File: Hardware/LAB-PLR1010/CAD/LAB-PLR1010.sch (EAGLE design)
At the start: 7 parts, among them U1 AD5270BRMZ-50, U2 LT3080EMS8EPBF

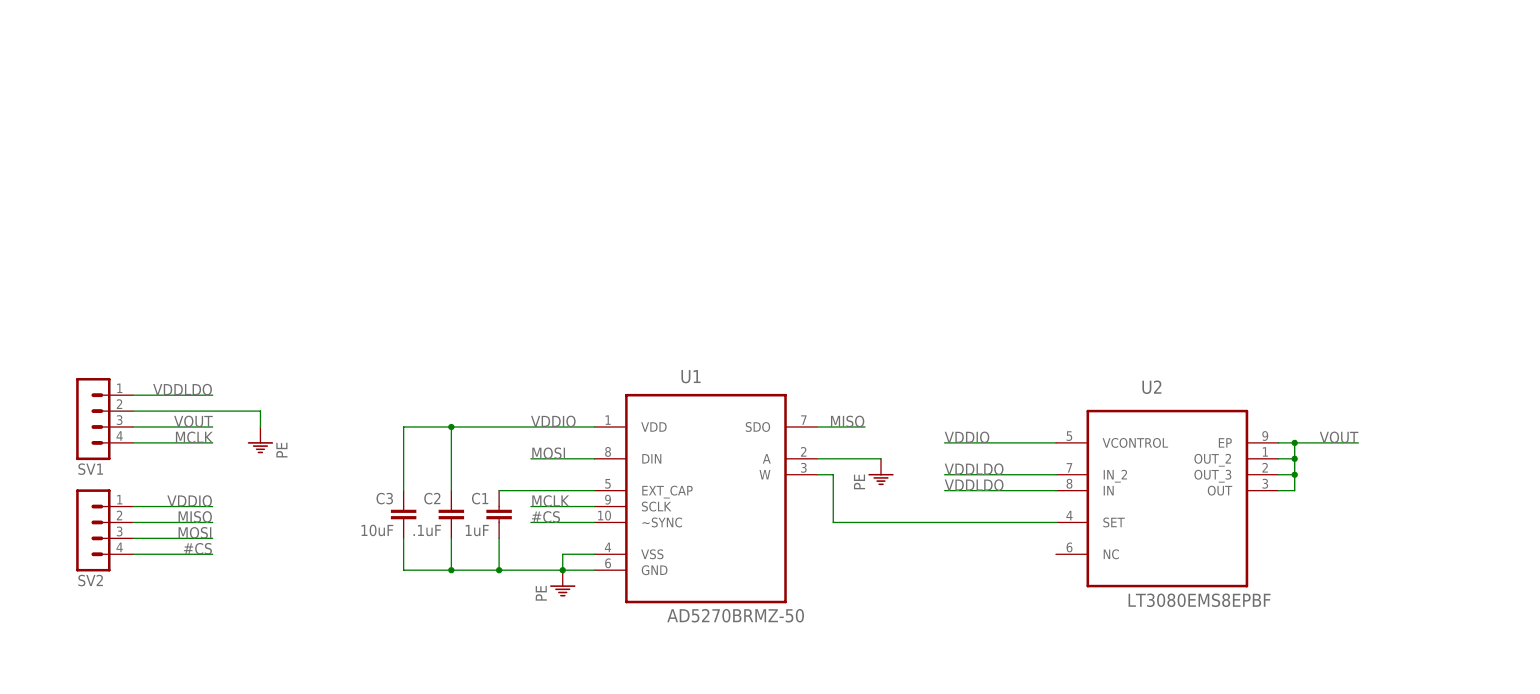
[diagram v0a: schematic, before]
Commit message: 1) Updates to the PLR1010 + datasheet and bills of materials
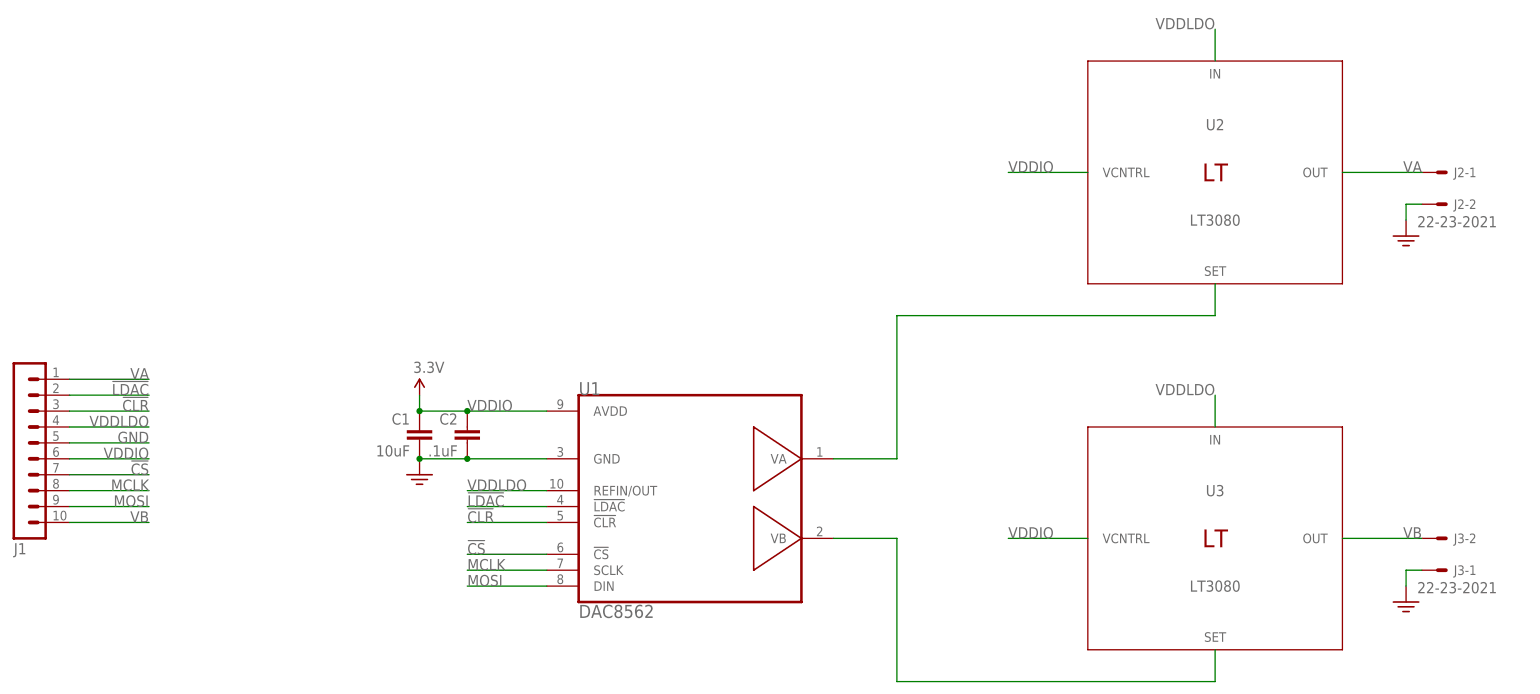
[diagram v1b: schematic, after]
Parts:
- removed C3: 10uF, SparkFun-Capacitors:1NF/1000PF-50V-10%(0603)
- removed SV1, SV2: (no value), LAB304:MA04-1
- added J1: (no value), con-lstb:MA10-1W
- added J2, J3: 22-23-2021, My Library-adm:22-23-2021
- added U3: LT3080, LAB-PLR1010:LT3080
- C1: value 1uF -> 10uF
- U1: value AD5270BRMZ-50 -> DAC8562; device Analog Devices_By_element14_Batch_1:AD5270BRMZ-50 -> LAB-PLR1010:DAC8562
- U2: value LT3080EMS8EPBF -> LT3080; device LAB-PLR1010:LT3080EMS8EPBF -> LAB-PLR1010:LT3080
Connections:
- removed net #CS: SV2.4, U1.~SYNC
- removed net MISO: SV2.2, U1.SDO
- removed net N$1: C1.1, U1.EXT_CAP
- removed net N$8: U1.W, U2.SET
- removed net PE: C1.2, C2.2, C3.2, SV1.2, U1.A, U1.GND, U1.VSS
- removed net VOUT: SV1.3, U2.EP, U2.OUT, U2.OUT_2, U2.OUT_3
- new net !CLR: J1.3, U1.!CLR
- new net !CS: J1.7, U1.!CS
- new net !LDAC: J1.2, U1.!LDAC
- new net GND: C1.2, C2.2, J1.5, J2-2.S, J3-1.S, U1.GND
- new net N$2: U1.VA, U2.SET
- new net N$3: U1.VB, U3.SET
- new net VA: J1.1, J2-1.S, U2.OUT
- new net VB: J1.10, J3-2.S, U3.OUT
- net MCLK: now also J1.8; no longer SV1.4
- net MOSI: now also J1.9; no longer SV2.3
- net VDDIO: now also C1.1, J1.6, U1.AVDD, U2.VCNTRL, U3.VCNTRL; no longer C3.1, SV2.1, U1.VDD, U2.VCONTROL
- net VDDLDO: now also J1.4, U1.REFIN/OUT, U3.IN; no longer SV1.1, U2.IN_2
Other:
- moved on the sheet: C1, C2
